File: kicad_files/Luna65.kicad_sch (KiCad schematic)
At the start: 332 parts, among them J1 TYPE-C-31-M12_13, J2 JSTPH, J3 uC Pin Headers, J4 nRF51 Pin Headers, J5 Pin Headers, Q1 DTC123JKAT146, Q2 AO3401A, SW0 SW_Push, SW1 Esc, SW10 9, SW11 0, SW12 -, SW13 =, SW14 BSP_200, SW15 Del, SW16 Tab_150, SW17 Q, SW18 W, SW19 E, SW2 1, SW20 R, SW21 T, SW22 Y, SW23 U, SW24 I, SW25 O, SW26 P, SW27 [, SW28 ], SW29 \_150, SW3 2, SW30 Home, SW31 Caps_175, SW32 A, SW33 S, SW34 D, SW35 F, SW36 G, SW37 H, SW38 J, SW39 K, SW4 3, SW40 L, SW41 ;, SW42 ', SW43 Ent_225, SW44 PgUp, SW45 LShft_225, SW46 Z, SW47 X, SW48 C, SW49 V, SW5 4, SW50 B, SW51 N, SW52 M, SW53 ,, SW54 ., SW55 /, SW56 RShft_175, SW57 Up, SW58 PgDn, SW59 LCtrl_125, SW6 5, SW60 Win_125, SW61 LAlt_125, SW62 Space_625, SW63 RAlt, SW64 Fn, SW65 RCtrl, SW66 Left, SW67 Down, SW68 Right, SW7 6, SW8 7, SW9 8, U1 ATMEGA32U4, U2 USBLC6-2SC6, U3 MCP73831, U4 AP2112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

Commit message: Rev 6 initial changes
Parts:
- removed C1, C8: 4.7nF, acheron_Components:C_0805_2012Metric, symbol Device:C_Small
- removed C10, C9: 10uF, acheron_Components:C_0805_2012Metric, symbol Device:C_Small
- removed C12: 1uF, acheron_Components:C_0805_2012Metric, symbol Device:C_Small
- removed C2: 0.1uF, acheron_Components:C_0805_2012Metric, symbol Device:C_Small
- removed D10, D11, D12, D13, D14, D15, D69, D9: 1N4148W, acheron_Components:D_SOD-123, symbol Device:D_Small
- removed D100, D101, D102, D103, D104, D105, D106, D107, D108, D109, D110, D111, D112, D113, D114, D115, D116, D117, D118, D119, D120, D121, D122, D123, D124, D125, D126, D127, D128, D129, D130, D131, D132, D133, D134, D135, D136, D137, D138, D71, D72, D73, D74, D75, D76, D77, D78, D79, D80, D81, D82, D83, D84, D85, D86, D87, D88, D89, D90, D91, D92, D93, D94, D95, D96, D97, D98, D99: LED_Small, LED_SMD:LED_1206_3216Metric_Pad1.42x1.75mm_HandSolder, symbol Device:LED_Small
- removed D139: Green, LED_SMD:LED_1206_3216Metric_Pad1.42x1.75mm_HandSolder, symbol Device:LED_Small
- removed D70: MBR120, acheron_Components:D_SOD-123, symbol Device:D_Schottky_Small
- removed H4: MountingHole, MountingHole:MountingHole_2.7mm_M2.5_Pad, symbol Mechanical:MountingHole_Pad
- removed J1: TYPE-C-31-M12_13, acheron_Connectors:TYPE-C-31-M-12, symbol acheronSymbols:TYPE-C-31-M12_13
- removed J2: JSTPH, Adafruit Feather 32u4 Bluefruit LE:JSTPH2, symbol Connector_Generic:Conn_01x02
- removed J5: Pin Headers, Connector_PinHeader_1.27mm:PinHeader_2x01_P1.27mm_Vertical, symbol Connector_Generic:Conn_01x02
- removed Q1: DTC123JKAT146, Package_TO_SOT_SMD:SOT-23, symbol acheronSymbols:DTC123J
- removed Q2: AO3401A, Package_TO_SOT_SMD:SOT-23, symbol Transistor_FET:AO3401A
- removed R1, R2: 5.1k, Resistor_SMD:R_0805_2012Metric_Pad1.20x1.40mm_HandSolder, symbol Device:R_Small
- removed R14: 1K, acheron_Components:R_SMD_1206, symbol Device:R
- removed R15: 100, acheron_Components:R_SMD_1206, symbol Device:R
- removed R3: 1M, Resistor_SMD:R_0805_2012Metric_Pad1.20x1.40mm_HandSolder, symbol Device:R_Small
- removed R4, R5: 22, Resistor_SMD:R_0805_2012Metric_Pad1.20x1.40mm_HandSolder, symbol Device:R_Small
- removed R6: 10K, Resistor_SMD:R_0805_2012Metric_Pad1.20x1.40mm_HandSolder, symbol Device:R_Small
- removed R7: 1K, Resistor_SMD:R_0805_2012Metric_Pad1.20x1.40mm_HandSolder, symbol Device:R_Small
- removed R8: 100K, Resistor_SMD:R_0805_2012Metric_Pad1.20x1.40mm_HandSolder, symbol Device:R_Small
- removed R83: 100, acheron_Components:R_SMD_1206, symbol Device:R_Small
- removed R9: 1M, acheron_Components:R_SMD_1206, symbol Device:R_Small
- removed SW10: 9, acheron_MXH:MX100H, symbol acheronSymbols:MXSwitch
- removed SW11: 0, acheron_MXH:MX100H, symbol acheronSymbols:MXSwitch
- removed SW12: -, acheron_MXH:MX100H, symbol acheronSymbols:MXSwitch
- removed SW13: =, acheron_MXH:MX100H, symbol acheronSymbols:MXSwitch
- removed SW14: BSP_200, acheron_MXH:MX200HR, symbol acheronSymbols:MXSwitch
- removed SW15: Del, acheron_MXH:MX100H, symbol acheronSymbols:MXSwitch
- removed SW24: I, acheron_MXH:MX100H, symbol acheronSymbols:MXSwitch
- removed SW25: O, acheron_MXH:MX100H, symbol acheronSymbols:MXSwitch
- removed SW26: P, acheron_MXH:MX100H, symbol acheronSymbols:MXSwitch
- removed SW27: [, acheron_MXH:MX100H, symbol acheronSymbols:MXSwitch
- removed SW28: ], acheron_MXH:MX100H, symbol acheronSymbols:MXSwitch
- removed SW29: \_150, acheron_MXH:MX150H, symbol acheronSymbols:MXSwitch
- removed SW30: Home, acheron_MXH:MX100H, symbol acheronSymbols:MXSwitch
- removed SW39: K, acheron_MXH:MX100H, symbol acheronSymbols:MXSwitch
- removed SW40: L, acheron_MXH:MX100H, symbol acheronSymbols:MXSwitch
- removed SW41: ;, acheron_MXH:MX100H, symbol acheronSymbols:MXSwitch
- removed SW42: ', acheron_MXH:MX100H, symbol acheronSymbols:MXSwitch
- removed SW43: Ent_225, acheron_MXH:MX225HR, symbol acheronSymbols:MXSwitch
- removed SW44: PgUp, acheron_MXH:MX100H, symbol acheronSymbols:MXSwitch
- removed SW52: M, acheron_MXH:MX100H, symbol acheronSymbols:MXSwitch
- removed SW53: ,, acheron_MXH:MX100H, symbol acheronSymbols:MXSwitch
- removed SW54: ., acheron_MXH:MX100H, symbol acheronSymbols:MXSwitch
- removed SW55: /, acheron_MXH:MX100H, symbol acheronSymbols:MXSwitch
- removed SW56: RShft_175, acheron_MXH:MX175H, symbol acheronSymbols:MXSwitch
- removed SW57: Up, acheron_MXH:MX100H, symbol acheronSymbols:MXSwitch
- removed SW58: PgDn, acheron_MXH:MX100H, symbol acheronSymbols:MXSwitch
- removed SW59: LCtrl_125, acheron_MXH:MX125H, symbol acheronSymbols:MXSwitch
- removed SW60: Win_125, acheron_MXH:MX125H, symbol acheronSymbols:MXSwitch
- removed SW61: LAlt_125, acheron_MXH:MX125H, symbol acheronSymbols:MXSwitch
- removed SW62: Space_625, acheron_MXH:MX625H, symbol acheronSymbols:MXSwitch
- removed SW63: RAlt, acheron_MXH:MX100H, symbol acheronSymbols:MXSwitch
- removed SW64: Fn, acheron_MXH:MX100H, symbol acheronSymbols:MXSwitch
- removed SW65: RCtrl, acheron_MXH:MX100H, symbol acheronSymbols:MXSwitch
- removed SW66: Left, acheron_MXH:MX100H, symbol acheronSymbols:MXSwitch
- removed SW67: Down, acheron_MXH:MX100H, symbol acheronSymbols:MXSwitch
- removed SW68: Right, acheron_MXH:MX100H, symbol acheronSymbols:MXSwitch
- removed SW9: 8, acheron_MXH:MX100H, symbol acheronSymbols:MXSwitch
- removed U2: USBLC6-2SC6, Package_TO_SOT_SMD:SOT-23-6, symbol Power_Protection:USBLC6-2SC6
- removed U3: MCP73831, Package_TO_SOT_SMD:SOT-23-5, symbol Battery_Management:MCP73831-2-OT
- removed U4: AP2112, Package_TO_SOT_SMD:SOT-23-5, symbol Regulator_Linear:SPX3819M5-L-3-3
- added C13, C14, C15, C16, C17, C18, C19, C20, C21, C22, C23, C24, C25, C26, C27, C28, C29, C30, C31, C32, C33, C34, C35, C36, C37, C38, C39, C40, C41, C42, C43, C44, C45, C46, C47, C48, C49, C50, C51, C52, C53, C54, C55, C56, C57, C58, C59, C60, C61, C62, C63, C64, C65, C66, C67, C68, C69, C70, C71, C72, C73, C74, C75, C76, C77, C78, C79, C80: 100n, acheron_Components:C_0805_2012Metric, symbol Device:C_Small
- added C81, C82: 100n, acheron_Components:C_0805_2012Metric, symbol Device:C
- added D100, D101, D102, D103, D104, D105, D106, D107, D108, D109, D110, D111, D112, D113, D114, D115, D116, D117, D118, D119, D120, D121, D122, D123, D124, D125, D126, D127, D128, D129, D130, D131, D132, D133, D134, D135, D136, D69, D70, D71, D72, D73, D74, D75, D76, D77, D78, D79, D80, D81, D82, D83, D84, D85, D86, D87, D88, D89, D90, D91, D92, D93, D94, D95, D96, D97, D98, D99: SK6812MINI-E, acheron_Components:SK6812MINI_3535_6028_3.2x2.8mm_Round, symbol acheron_Symbols:SK6812MINI-E
- added D59, D60, D61, D62, D63, D64, D65: 1N4148W, acheron_Components:D_SOD-123, symbol Device:D_Small
- added H4: MountingHole, MountingHole:MountingHole_2.7mm_M2.5_Pad, symbol Mechanical:MountingHole
- added J1: Molex Power, Luna65:MOLEX_78171-0005, symbol Connector_Generic:Conn_01x05
- added R14, R15: 5.1R, acheron_Components:C_0805_2012Metric, symbol Device:R_Small
- added SW24, SW25, SW26, SW27, SW28, SW30, SW32, SW33, SW34, SW35, SW36, SW37, SW38, SW39, SW40, SW41, SW42, SW44, SW53, SW54, SW55, SW57, SW58, SW63, SW64, SW65, SW66, SW67, SW68: Mechanical_Switch, acheron_MXH_metalrings:MX100H, symbol acheron_Symbols:Mechanical_Switch
- added SW29: Mechanical_Switch, acheron_MXH_metalrings:MX150H, symbol acheron_Symbols:Mechanical_Switch
- added SW31, SW56: Mechanical_Switch, acheron_MXH_metalrings:MX175H, symbol acheron_Symbols:Mechanical_Switch
- added SW43: Mechanical_Switch, acheron_MXH_metalrings:MX225H, symbol acheron_Symbols:Mechanical_Switch
- added SW59, SW60, SW61: Mechanical_Switch, acheron_MXH_metalrings:MX125H, symbol acheron_Symbols:Mechanical_Switch
- added SW62: Mechanical_Switch, acheron_MXH_metalrings:MX625HR, symbol acheron_Symbols:Mechanical_Switch
- added U3: TXS0101DBVR, acheron_Components:SOT-23-6, symbol acheronSymbols:TXS0101
- J2: renamed from J3; footprint Connector_PinHeader_1.27mm:PinHeader_2x03_P1.27mm_Vertical -> Connector_PinHeader_2.54mm:PinHeader_2x03_P2.54mm_Vertical
- J3: renamed from J4; footprint Connector_PinHeader_1.27mm:PinHeader_2x03_P1.27mm_Vertical -> Connector_PinHeader_2.54mm:PinHeader_2x03_P2.54mm_Vertical
- R16, R17, R18, R19, R20, R21, R22, R23, R24, R25, R26, R27, R28, R29, R30, R31, R32, R33, R34, R35, R36, R37, R38, R39, R40, R41, R42, R43, R44, R45, R46, R47, R48, R49, R50, R51, R52, R53, R54, R55, R56, R57, R58, R59, R60, R61, R62, R63, R64, R65, R66, R67, R68, R69, R70, R71, R72, R73, R74, R75, R76, R77, R78, R79, R80, R81: value 100 -> 5.1R; footprint acheron_Components:R_SMD_1206 -> acheron_Components:C_0805_2012Metric; Package (none) -> R0402
- R82: value 100 -> 10k; footprint acheron_Components:R_SMD_1206 -> Resistor_SMD:R_0805_2012Metric_Pad1.20x1.40mm_HandSolder; Package (none) -> R0805
- SW1: value Esc -> Mechanical_Switch; footprint acheron_MXH:MX100H -> acheron_MXH_metalrings:MX100H; symbol acheronSymbols:MXSwitch -> acheron_Symbols:Mechanical_Switch; Keycode (none) -> ESC
- SW10: renamed from SW46; value Z -> Mechanical_Switch; footprint acheron_MXH:MX100H -> acheron_MXH_metalrings:MX100H; symbol acheronSymbols:MXSwitch -> acheron_Symbols:Mechanical_Switch; Keycode (none) -> 9
- SW11: renamed from SW47; value X -> Mechanical_Switch; footprint acheron_MXH:MX100H -> acheron_MXH_metalrings:MX100H; symbol acheronSymbols:MXSwitch -> acheron_Symbols:Mechanical_Switch; Keycode (none) -> 0
- SW12: renamed from SW48; value C -> Mechanical_Switch; footprint acheron_MXH:MX100H -> acheron_MXH_metalrings:MX100H; symbol acheronSymbols:MXSwitch -> acheron_Symbols:Mechanical_Switch; Keycode (none) -> -
- SW13: renamed from SW49; value V -> Mechanical_Switch; footprint acheron_MXH:MX100H -> acheron_MXH_metalrings:MX100H; symbol acheronSymbols:MXSwitch -> acheron_Symbols:Mechanical_Switch; Keycode (none) -> =
- SW14: renamed from SW50; value B -> Mechanical_Switch; footprint acheron_MXH:MX100H -> acheron_MXH_metalrings:MX200H; symbol acheronSymbols:MXSwitch -> acheron_Symbols:Mechanical_Switch; Keycode (none) -> BSPC
- SW15: renamed from SW51; value N -> Mechanical_Switch; footprint acheron_MXH:MX100H -> acheron_MXH_metalrings:MX100H; symbol acheronSymbols:MXSwitch -> acheron_Symbols:Mechanical_Switch; Keycode (none) -> HOME
- SW16: value Tab_150 -> Mechanical_Switch; footprint acheron_MXH:MX150H -> acheron_MXH_metalrings:MX150H; symbol acheronSymbols:MXSwitch -> acheron_Symbols:Mechanical_Switch; Keycode (none) -> TAB
- SW17: value Q -> Mechanical_Switch; footprint acheron_MXH:MX100H -> acheron_MXH_metalrings:MX100H; symbol acheronSymbols:MXSwitch -> acheron_Symbols:Mechanical_Switch; Keycode (none) -> Q
- SW18: value W -> Mechanical_Switch; footprint acheron_MXH:MX100H -> acheron_MXH_metalrings:MX100H; symbol acheronSymbols:MXSwitch -> acheron_Symbols:Mechanical_Switch; Keycode (none) -> W
- SW19: value E -> Mechanical_Switch; footprint acheron_MXH:MX100H -> acheron_MXH_metalrings:MX100H; symbol acheronSymbols:MXSwitch -> acheron_Symbols:Mechanical_Switch; Keycode (none) -> E
- SW2: value 1 -> Mechanical_Switch; footprint acheron_MXH:MX100H -> acheron_MXH_metalrings:MX100H; symbol acheronSymbols:MXSwitch -> acheron_Symbols:Mechanical_Switch; Keycode (none) -> 1
- SW20: value R -> Mechanical_Switch; footprint acheron_MXH:MX100H -> acheron_MXH_metalrings:MX100H; symbol acheronSymbols:MXSwitch -> acheron_Symbols:Mechanical_Switch; Keycode (none) -> R
- SW21: value T -> Mechanical_Switch; footprint acheron_MXH:MX100H -> acheron_MXH_metalrings:MX100H; symbol acheronSymbols:MXSwitch -> acheron_Symbols:Mechanical_Switch; Keycode (none) -> T
- SW22: value Y -> Mechanical_Switch; footprint acheron_MXH:MX100H -> acheron_MXH_metalrings:MX100H; symbol acheronSymbols:MXSwitch -> acheron_Symbols:Mechanical_Switch; Keycode (none) -> Y
- SW23: value U -> Mechanical_Switch; footprint acheron_MXH:MX100H -> acheron_MXH_metalrings:MX100H; symbol acheronSymbols:MXSwitch -> acheron_Symbols:Mechanical_Switch; Keycode (none) -> U
- SW3: value 2 -> Mechanical_Switch; footprint acheron_MXH:MX100H -> acheron_MXH_metalrings:MX100H; symbol acheronSymbols:MXSwitch -> acheron_Symbols:Mechanical_Switch; Keycode (none) -> 2
- SW4: value 3 -> Mechanical_Switch; footprint acheron_MXH:MX100H -> acheron_MXH_metalrings:MX100H; symbol acheronSymbols:MXSwitch -> acheron_Symbols:Mechanical_Switch; Keycode (none) -> 3
- SW45: renamed from SW31; value Caps_175 -> Mechanical_Switch; footprint acheron_MXH:MX175H -> acheron_MXH_metalrings:MX225H; symbol acheronSymbols:MXSwitch -> acheron_Symbols:Mechanical_Switch; Keycode (none) -> LSHFT
- SW46: renamed from SW32; value A -> Mechanical_Switch; footprint acheron_MXH:MX100H -> acheron_MXH_metalrings:MX100H; symbol acheronSymbols:MXSwitch -> acheron_Symbols:Mechanical_Switch; Keycode (none) -> Z
- SW47: renamed from SW33; value S -> Mechanical_Switch; footprint acheron_MXH:MX100H -> acheron_MXH_metalrings:MX100H; symbol acheronSymbols:MXSwitch -> acheron_Symbols:Mechanical_Switch; Keycode (none) -> X
- SW48: renamed from SW34; value D -> Mechanical_Switch; footprint acheron_MXH:MX100H -> acheron_MXH_metalrings:MX100H; symbol acheronSymbols:MXSwitch -> acheron_Symbols:Mechanical_Switch; Keycode (none) -> C
- SW49: renamed from SW35; value F -> Mechanical_Switch; footprint acheron_MXH:MX100H -> acheron_MXH_metalrings:MX100H; symbol acheronSymbols:MXSwitch -> acheron_Symbols:Mechanical_Switch; Keycode (none) -> V
- SW5: value 4 -> Mechanical_Switch; footprint acheron_MXH:MX100H -> acheron_MXH_metalrings:MX100H; symbol acheronSymbols:MXSwitch -> acheron_Symbols:Mechanical_Switch; Keycode (none) -> 4
- SW50: renamed from SW36; value G -> Mechanical_Switch; footprint acheron_MXH:MX100H -> acheron_MXH_metalrings:MX100H; symbol acheronSymbols:MXSwitch -> acheron_Symbols:Mechanical_Switch; Keycode (none) -> B
- SW51: renamed from SW37; value H -> Mechanical_Switch; footprint acheron_MXH:MX100H -> acheron_MXH_metalrings:MX100H; symbol acheronSymbols:MXSwitch -> acheron_Symbols:Mechanical_Switch; Keycode (none) -> N
- SW52: renamed from SW38; value J -> Mechanical_Switch; footprint acheron_MXH:MX100H -> acheron_MXH_metalrings:MX100H; symbol acheronSymbols:MXSwitch -> acheron_Symbols:Mechanical_Switch; Keycode (none) -> M
- SW6: value 5 -> Mechanical_Switch; footprint acheron_MXH:MX100H -> acheron_MXH_metalrings:MX100H; symbol acheronSymbols:MXSwitch -> acheron_Symbols:Mechanical_Switch; Keycode (none) -> 5
- SW7: value 6 -> Mechanical_Switch; footprint acheron_MXH:MX100H -> acheron_MXH_metalrings:MX100H; symbol acheronSymbols:MXSwitch -> acheron_Symbols:Mechanical_Switch; Keycode (none) -> 6
- SW8: value 7 -> Mechanical_Switch; footprint acheron_MXH:MX100H -> acheron_MXH_metalrings:MX100H; symbol acheronSymbols:MXSwitch -> acheron_Symbols:Mechanical_Switch; Keycode (none) -> 7
- SW9: renamed from SW45; value LShft_225 -> Mechanical_Switch; footprint acheron_MXH:MX225HR -> acheron_MXH_metalrings:MX100H; symbol acheronSymbols:MXSwitch -> acheron_Symbols:Mechanical_Switch; Keycode (none) -> 8
- Y1: value 8MHz -> 16MHz
- renumbered C13 to C11, D60 to D10, D61 to D11, D62 to D12, D63 to D13, D140 to D137, D141 to D138, D64 to D14, D65 to D15, D59 to D9, U5 to U2
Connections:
- net LED_PWM is gone; now on net Row1: U1.18 (PD0/SCL/~{INT0})
- net VBUS is gone; now on net 5V: U1.7 (VBUS)
- net 3.3V: now also J2.5 (Pin_5), R82.1, C81.2, J1.1 (Pin_1), U3.1 (VCCA); no longer J2.2 (Pin_2)
- net Col1: now also U1.26 (ADC9/T1/PD6), SW31.1, SW59.1; no longer SW9.1 (Col), U1.36 (ADC7/PF7)
- net Col10: now also SW10.1, U1.38 (ADC5/PF5), SW25.1, SW40.1, SW54.1, SW58.1, SW64.1; no longer U1.31 (PC6)
- net Col11: now also SW11.1, U1.39 (ADC4/PF4), SW26.1, SW41.1, SW55.1, SW65.1, SW68.1; no longer U1.30 (PCINT6/ADC13/PB6)
- net Col12: now also SW12.1, U1.40 (ADC1/PF1), SW27.1, SW42.1, SW56.1, SW66.1, SW67.1; no longer U1.29 (PCINT4/ADC12/PB5)
- net Col2: now also U1.27 (ADC10/T0/PD7), SW32.1, SW60.1; no longer SW10.1 (Col), U1.19 (PD1/SDA/~{INT1})
- net Col3: now also U1.28 (ADC4/PCINT11/PB4), SW33.1, SW61.1; no longer SW11.1 (Col), U1.20 (PD2/RDX1/~{INT2})
- net Col4: now also U1.29 (PCINT4/ADC12/PB5), SW34.1, SW62.1; no longer SW12.1 (Col), U1.21 (PD3/TXD1/~{INT3})
- net Col5: now also U1.30 (PCINT6/ADC13/PB6), SW35.1, SW43.1, SW44.1; no longer SW13.1 (Col), U1.22 (PD5/~{CTS}/XCK1)
- net Col6: now also SW15.1, U1.31 (PC6), SW30.1, SW36.1; no longer SW14.1 (Col), U1.26 (ADC9/T1/PD6)
- net Col7: now also SW14.1, U1.32 (CLK/PC7), SW29.1, SW37.1; no longer SW15.1 (Col), U1.27 (ADC10/T0/PD7)
- net Col8: now also SW13.1, U1.36 (ADC7/PF7), SW28.1, SW38.1; no longer U1.12 (PB7/RTS)
- net Col9: now also SW9.1, U1.37 (ADC6/PF6), SW24.1, SW39.1, SW53.1, SW57.1, SW63.1; no longer U1.32 (CLK/PC7)
- net D+: now also J1.4 (Pin_4)
- net D-: now also J1.3 (Pin_3)
- net GND: now also C13.2, C14.2, C15.2, C16.2, C17.2, C18.2, C19.2, C20.2, C21.2, C22.2, C23.2, C24.2, C25.2, C26.2, C27.2, C28.2, C29.2, C30.2, C31.2, C32.2, C33.2, C34.2, C35.2, C36.2, C37.2, C38.2, C39.2, C40.2, C41.2, C42.2, C43.2, C44.2, C45.2, C46.2, C47.2, C48.2, C49.2, C50.2, C51.2, C52.2, C53.2, C54.2, C55.2, C56.2, C57.2, C58.2, C59.2, C60.2, C61.2, C62.2, C63.2, C64.2, C65.2, C66.2, C67.2, C68.2, C69.2, C70.2, C71.2, C72.2, C73.2, C74.2, C75.2, C76.2, C77.2, C78.2, C79.2, C80.2, C81.1, C82.2, D100.3 (VSS), D101.3 (VSS), D102.3 (VSS), D103.3 (VSS), D104.3 (VSS), D105.3 (VSS), D106.3 (VSS), D107.3 (VSS), D108.3 (VSS), D109.3 (VSS), D110.3 (VSS), D111.3 (VSS), D112.3 (VSS), D113.3 (VSS), D114.3 (VSS), D115.3 (VSS), D116.3 (VSS), D117.3 (VSS), D118.3 (VSS), D119.3 (VSS), D120.3 (VSS), D121.3 (VSS), D122.3 (VSS), D123.3 (VSS), D124.3 (VSS), D125.3 (VSS), D126.3 (VSS), D127.3 (VSS), D128.3 (VSS), D129.3 (VSS), D130.3 (VSS), D131.3 (VSS), D132.3 (VSS), D133.3 (VSS), D134.3 (VSS), D135.3 (VSS), D136.3 (VSS), D69.3 (VSS), D70.3 (VSS), D71.3 (VSS), D72.3 (VSS), D73.3 (VSS), D74.3 (VSS), D75.3 (VSS), D76.3 (VSS), D77.3 (VSS), D78.3 (VSS), D79.3 (VSS), D80.3 (VSS), D81.3 (VSS), D82.3 (VSS), D83.3 (VSS), D84.3 (VSS), D85.3 (VSS), D86.3 (VSS), D87.3 (VSS), D88.3 (VSS), D89.3 (VSS), D90.3 (VSS), D91.3 (VSS), D92.3 (VSS), D93.3 (VSS), D94.3 (VSS), D95.3 (VSS), D96.3 (VSS), D97.3 (VSS), D98.3 (VSS), D99.3 (VSS), J1.5 (Pin_5), U3.2 (GND)
- net MISO: now also J2.3 (Pin_3); no longer J2.1 (Pin_1)
- net MOSI: now also J2.1 (Pin_1); no longer J2.4 (Pin_4)
- net RESET: now also J2.2 (Pin_2); no longer J2.5 (Pin_5)
- net Row1: now also D10.1 (K), D11.1 (K), D12.1 (K), D9.1 (K); no longer U1.41 (ADC0/PF0)
- net Row2: now also U1.19 (PD1/SDA/~{INT1}); no longer U1.40 (ADC1/PF1)
- net Row3: now also U1.20 (PD2/RDX1/~{INT2}); no longer U1.39 (ADC4/PF4)
- net Row4: now also U1.22 (PD5/~{CTS}/XCK1); no longer U1.38 (ADC5/PF5)
- net Row5: now also D28.1 (K), D29.1 (K), D30.1 (K), D43.1 (K), U1.21 (PD3/TXD1/~{INT3}), D59.1 (K), D60.1 (K), D61.1 (K), D62.1 (K), D63.1 (K), D64.1 (K), D65.1 (K); no longer D10.1 (K), D11.1 (K), D12.1 (K), D13.1 (K), D14.1 (K), D15.1 (K), D44.1 (K), D58.1 (K), D67.1 (K), D68.1 (K), D9.1 (K), U1.37 (ADC6/PF6)
- net Row6: now also D13.1 (K), D14.1 (K), D15.1 (K), D44.1 (K), D58.1 (K), D67.1 (K), D68.1 (K), U1.41 (ADC0/PF0); no longer D28.1 (K), D29.1 (K), D30.1 (K), D43.1 (K), U1.28 (ADC4/PCINT11/PB4)
- net SCK: now also J2.4 (Pin_4); no longer J2.3 (Pin_3)
- net at SW14.2: now also D14.2 (A); no longer D50.2 (A)
- net 5V: now reaches R73.2
- net 5V: now also R16.2, R17.2, R18.2, R19.2, R20.2, R21.2, R22.2, R23.2, R24.2, R25.2, R26.2, R27.2, R28.2, R29.2, R30.2, R31.2, R32.2, R33.2, R34.2, R35.2, R36.2, R37.2, R38.2, R39.2, R40.2, R41.2, R42.2, R43.2, R44.2, R45.2, R46.2, R47.2, R48.2, R49.2, R50.2, R51.2, R52.2, R53.2, R54.2, R55.2, R56.2, R57.2, R58.2, R59.2, R60.2, R61.2, R62.2, R63.2, R64.2, R65.2, R66.2, R67.2, R68.2, R69.2, R70.2, R71.2, R72.2, R74.2, R75.2, R76.2, R77.2, R78.2, R79.2, R80.2, R81.2, C82.1, J1.2 (Pin_2), R14.2, R15.2, U3.6 (VCCB)
- net at SW52.2: now also D52.2 (A); no longer D38.2 (A)
- net at D42.2 (A): now also SW42.2
- net at D58.2 (A): now also SW58.2
- net at SW50.2: now also D50.2 (A); no longer D36.2 (A)
- net at SW10.2: now also D10.2 (A); no longer D46.2 (A)
- net at R82.2: now also U3.5 (OE)
- net at D15.2 (A): now also SW15.2
- net at D12.2 (A): now also SW12.2
- net at D31.2 (A): now also SW31.2; no longer SW45.2 (Row)
- net at D66.2 (A): now also SW66.2
- net at D26.2 (A): now also SW26.2
- net at SW48.2: now also D48.2 (A); no longer D34.2 (A)
- net at D43.2 (A): now also SW43.2
- net at SW51.2: now also D51.2 (A); no longer D37.2 (A)
- net at D55.2 (A): now also SW55.2
- net at D40.2 (A): now also SW40.2
- net at D25.2 (A): now also SW25.2
- net at D67.2 (A): now also SW67.2
- net at D30.2 (A): now also SW30.2
- net at SW46.2: now also D46.2 (A); no longer D32.2 (A)
- net at D11.2 (A): now also SW11.2
- net at D29.2 (A): now also SW29.2
- net at D49.2 (A): now also SW49.2; no longer SW13.2 (Row)
- net at D54.2 (A): now also SW54.2
- net at D47.2 (A): now also SW47.2; no longer SW11.2 (Row)
- net at D9.2 (A): now also SW9.2
- net at D13.2 (A): now also SW13.2
- net at D28.2 (A): now also SW28.2
- net at D35.2 (A): now also SW35.2; no longer SW49.2 (Row)
- net at D53.2 (A): now also SW53.2
- net at D68.2 (A): now also SW68.2
- net at D45.2 (A): now also SW45.2; no longer SW9.2 (Row)
- net at D24.2 (A): now also SW24.2
- net at D39.2 (A): now also SW39.2
- net at D44.2 (A): now also SW44.2
- net at D27.2 (A): now also SW27.2
- net at D57.2 (A): now also SW57.2
- net at D56.2 (A): now also SW56.2
- net at D41.2 (A): now also SW41.2
- net at D33.2 (A): now also SW33.2; no longer SW47.2 (Row)
- new net: C21.1, D77.1 (VDD), R22.1
- new net: C13.1, D69.1 (VDD), R14.1
- new net: C41.1, D97.1 (VDD), R42.1
- new net: C52.1, D108.1 (VDD), R53.1
- new net: C33.1, D89.1 (VDD), R34.1
- new net: D60.2 (A), SW60.2
- new net: C67.1, D123.1 (VDD), R68.1
- new net: D119.4 (DIN), D123.2 (DOUT)
- new net: D123.4 (DIN), D127.2 (DOUT)
- new net: C64.1, D120.1 (VDD), R65.1
- new net: C28.1, D84.1 (VDD), R29.1
- new net: C16.1, D72.1 (VDD), R17.1
- new net: C42.1, D98.1 (VDD), R43.1
- new net: C15.1, D129.1 (VDD), R16.1
- new net: D65.2 (A), SW65.2
- new net: C26.1, D82.1 (VDD), R27.1
- new net: D82.2 (DOUT), D87.4 (DIN)
- new net: D77.2 (DOUT), D82.4 (DIN)
- new net: C74.1, D130.1 (VDD), R75.1
- new net: C69.1, D116.1 (VDD), R70.1
- new net: D111.4 (DIN), D116.2 (DOUT)
- new net: D116.4 (DIN), D121.2 (DOUT)
- new net: D84.4 (DIN), D89.2 (DOUT)
- new net: D89.4 (DIN), D94.2 (DOUT)
- new net: C37.1, D93.1 (VDD), R38.1
- new net: C32.1, D88.1 (VDD), R33.1
- new net: D83.4 (DIN), D88.2 (DOUT)
- new net: D88.4 (DIN), D93.2 (DOUT)
- new net: C55.1, D101.1 (VDD), R56.1
- new net: D101.2 (DOUT), D96.4 (DIN)
- new net: D101.4 (DIN), D106.2 (DOUT)
- new net: D62.2 (A), SW62.2
- new net: C36.1, D92.1 (VDD), R37.1
- new net: D63.2 (A), SW63.2
- new net: C73.1, D121.1 (VDD), R74.1
- new net: C35.1, D81.1 (VDD), R36.1
- new net: C66.1, D122.1 (VDD), R67.1
- new net: C54.1, D110.1 (VDD), R55.1
- new net: C57.1, D113.1 (VDD), R58.1
- new net: C40.1, D86.1 (VDD), R41.1
- new net: D81.4 (DIN), D86.2 (DOUT)
- new net: D86.4 (DIN), D91.2 (DOUT)
- new net: D92.2 (DOUT), D97.4 (DIN)
- new net: D87.2 (DOUT), D92.4 (DIN)
- new net: D64.2 (A), SW64.2
- new net: D59.2 (A), SW59.2
- new net: C75.1, D131.1 (VDD), R76.1
- new net: D127.4 (DIN), D131.2 (DOUT)
- new net: D131.4 (DIN), D135.2 (DOUT)
- new net: C18.1, D74.1 (VDD), R19.1
- new net: C61.1, D117.1 (VDD), R62.1
- new net: C49.1, D105.1 (VDD), R50.1
- new net: D105.2 (DOUT), D110.4 (DIN)
- new net: D100.2 (DOUT), D105.4 (DIN)
- new net: C76.1, D132.1 (VDD), R77.1
- new net: C65.1, D111.1 (VDD), R66.1
- new net: D106.4 (DIN), D111.2 (DOUT)
- new net: C70.1, D126.1 (VDD), R71.1
- new net: C38.1, D94.1 (VDD), R39.1
- new net: C51.1, D107.1 (VDD), R52.1
- new net: D107.2 (DOUT), D112.4 (DIN)
- new net: D102.2 (DOUT), D107.4 (DIN)
- new net: C22.1, D78.1 (VDD), R23.1
- new net: C59.1, D115.1 (VDD), R60.1
- new net: D69.4 (DIN), D74.2 (DOUT)
- new net: D74.4 (DIN), D79.2 (DOUT)
- new net: C45.1, D91.1 (VDD), R46.1
- new net: D110.2 (DOUT), D115.4 (DIN)
- new net: D61.2 (A), SW61.2
- new net: D120.2 (DOUT), D124.4 (DIN)
- new net: D115.2 (DOUT), D120.4 (DIN)
- new net: D129.2 (DOUT), D70.4 (DIN)
- new net: D129.4 (DIN), D133.2 (DOUT)
- new net: C58.1, D114.1 (VDD), R59.1
- new net: D94.4 (DIN), D99.2 (DOUT)
- new net: C27.1, D83.1 (VDD), R28.1
- new net: C60.1, D106.1 (VDD), R61.1
- new net: D122.2 (DOUT), D126.4 (DIN)
- new net: D117.2 (DOUT), D122.4 (DIN)
- new net: C47.1, D103.1 (VDD), R48.1
- new net: C56.1, D112.1 (VDD), R57.1
- new net: C17.1, D73.1 (VDD), R18.1
- new net: C79.1, D135.1 (VDD), R80.1
- new net: C25.1, D71.1 (VDD), R26.1
- new net: C78.1, D134.1 (VDD), R79.1
- new net: C23.1, D79.1 (VDD), R24.1
- new net: D79.4 (DIN), D84.2 (DOUT)
- new net: C44.1, D100.1 (VDD), R45.1
- new net: D100.4 (DIN), D95.2 (DOUT)
- new net: D135.4 (DIN), D136.2 (DOUT)
- new net: D72.2 (DOUT), D77.4 (DIN)
- new net: D72.4 (DIN), D73.2 (DOUT)
- new net: C63.1, D119.1 (VDD), R64.1
- new net: C48.1, D104.1 (VDD), R49.1
- new net: C77.1, D125.1 (VDD), R78.1
- new net: D121.4 (DIN), D125.2 (DOUT)
- new net: D125.4 (DIN), D134.2 (DOUT)
- new net: C39.1, D95.1 (VDD), R40.1
- new net: C20.1, D133.1 (VDD), R21.1
- new net: D133.4 (DIN), D71.2 (DOUT)
- new net: D36.2 (A), SW36.2
- new net: D112.2 (DOUT), D117.4 (DIN)
- new net: D93.4 (DIN), D98.2 (DOUT)
- new net: D103.2 (DOUT), D98.4 (DIN)
- new net: D37.2 (A), SW37.2
- new net: D102.4 (DIN), D97.2 (DOUT)
- new net: D132.2 (DOUT), D136.4 (DIN)
- new net: D128.2 (DOUT), D132.4 (DIN)
- new net: D109.4 (DIN), D114.2 (DOUT)
- new net: D114.4 (DIN), D119.2 (DOUT)
- new net: D73.4 (DIN), D78.2 (DOUT)
- new net: D38.2 (A), SW38.2
- new net: D130.2 (DOUT), D134.4 (DIN)
- new net: D126.2 (DOUT), D130.4 (DIN)
- new net: C46.1, D102.1 (VDD), R47.1
- new net: C71.1, D127.1 (VDD), R72.1
- new net: C50.1, D96.1 (VDD), R51.1
- new net: C62.1, D118.1 (VDD), R63.1
- new net: D103.4 (DIN), D108.2 (DOUT)
- new net: D78.4 (DIN), D83.2 (DOUT)
- new net: C53.1, D109.1 (VDD), R54.1
- new net: D108.4 (DIN), D113.2 (DOUT)
- new net: D34.2 (A), SW34.2
- new net: C72.1, D128.1 (VDD), R73.1
- new net: C24.1, D80.1 (VDD), R25.1
- new net: D104.2 (DOUT), D99.4 (DIN)
- new net: D104.4 (DIN), D109.2 (DOUT)
- new net: C80.1, D136.1 (VDD), R81.1
- new net: C14.1, D70.1 (VDD), R15.1
- new net: D90.2 (DOUT), D95.4 (DIN)
- new net: C68.1, D124.1 (VDD), R69.1
- new net: C43.1, D99.1 (VDD), R44.1
- new net: C31.1, D87.1 (VDD), R32.1
- new net: D113.4 (DIN), D118.2 (DOUT)
- new net: D76.4 (DIN), D81.2 (DOUT)
- new net: D91.4 (DIN), D96.2 (DOUT)
- new net: C29.1, D85.1 (VDD), R30.1
- new net: D85.2 (DOUT), D90.4 (DIN)
- new net: D80.2 (DOUT), D85.4 (DIN)
- new net: D70.2 (DOUT), D75.4 (DIN)
- new net: C30.1, D76.1 (VDD), R31.1
- new net: D71.4 (DIN), D76.2 (DOUT)
- new net: C19.1, D75.1 (VDD), R20.1
- new net: D124.2 (DOUT), D128.4 (DIN)
- new net: D75.2 (DOUT), D80.4 (DIN)
- new net: C34.1, D90.1 (VDD), R35.1
- new net: D32.2 (A), SW32.2
- new net RGB_3V3: U1.12 (PB7/RTS), U3.3 (A)
- new net RGB_5V: D118.4 (DIN), U3.4 (B)
- no-connect marks 4 -> 2
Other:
- note added: "'"
- note added: ","
- note added: "-"
- note added: "."
- note added: "/"
- note added: "0"
- note added: "16 February 2022"
- note added: "2"
- note added: "3"
- note added: "4"
- note added: "6"
- note added: "7"
- note added: "8"
- note added: "9"
- note added: ":"
- note added: "="
- note added: "A"
- note added: "B"
- note added: "BKSP"
- note added: "C"
- note added: "CAPS"
- note added: "D"
- note added: "DOWN"
- note added: "Daughter-board connector"
- note added: "E"
- note added: "END"
- note added: "ENT"
- note added: "ESC"
- note added: "F"
- note added: "FN"
- note added: "G"
- note added: "H"
- note added: "HOME"
- note added: "I"
- note added: "J"
- note added: "K"
- note added: "L"
- note added: "LALT"
- note added: "LCTRL"
- note added: "LEFT"
- note added: "LSHFT"
- note added: "M"
- note added: "N"
- note added: "O"
- note added: "P"
- note added: "PGDN"
- note added: "PGUP"
- note added: "Pin Headers"
- note added: "Q"
- note added: "R"
- note added: "RALT"
- note added: "RCTRL"
- note added: "RGB Level Shifter"
- note added: "RGB Matrix"
- note added: "RIGHT"
- note added: "RSHFT"
- note added: "S"
- note added: "SPACE"
- note added: "T"
- note added: "TAB"
- note added: "U"
- note added: "UP"
- note added: "V"
- note added: "W"
- note added: "WIN"
- note added: "X"
- note added: "Y"
- note added: "Z"
- note added: "["
- note added: "\"
- note added: "]"
- note removed: "3.3V LDO Regulator"
- note removed: "7 December 2021"
- note removed: "CASE to GND"
- note removed: "LED Matrix"
- note removed: "LiPo Charge Controller"
- note removed: "Shield"
- note removed: "USB ESD Protection"
- note removed: "USB-C Receptacle"
- moved on the sheet: C11, C3, C4, C5, C6, C7, D1, D10, D11, D12, D13, D137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

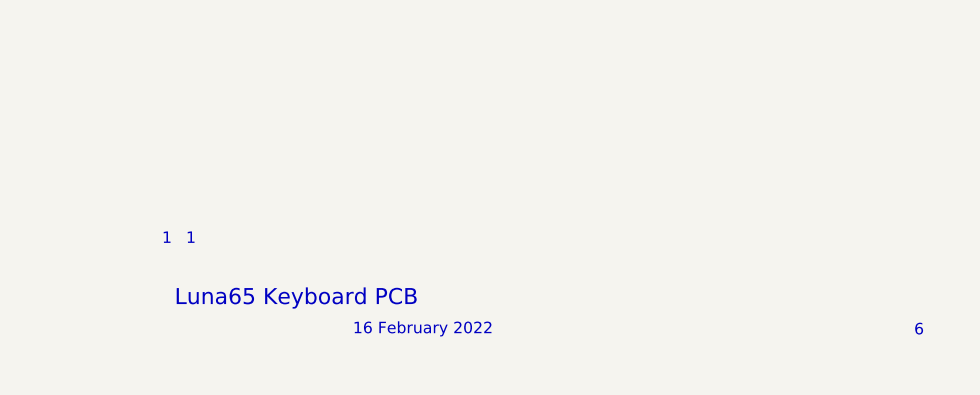
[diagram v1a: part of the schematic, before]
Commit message: DB Rev C
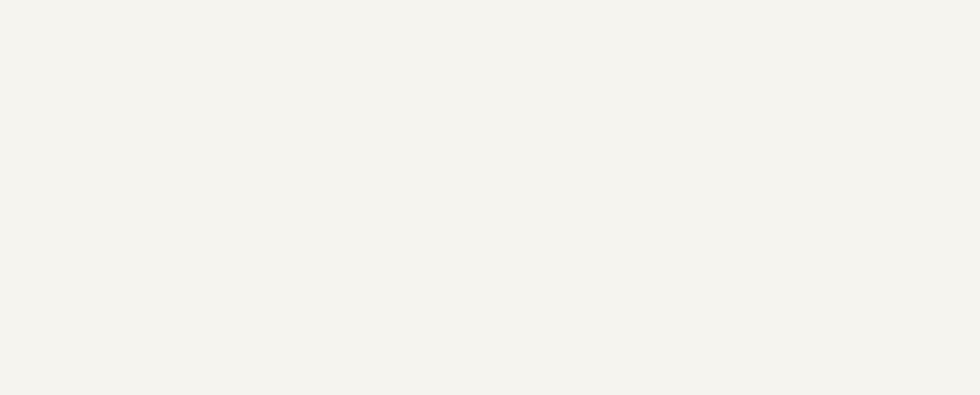
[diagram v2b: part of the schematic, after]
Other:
- note removed: "16 February 2022"
- note removed: "Luna65 Keyboard PCB"
- company: (none) -> Neil Khera
- title: (none) -> Luna65 Keyboard PCB
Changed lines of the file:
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@@
 (kicad_sch (version 20211123) (generator eeschema)
   (paper "User" 799.998 264.998)
+  (title_block
+    (title "Luna65 Keyboard PCB")
+    (date "2022-03-04")
+    (rev "6")
+    (company "Neil Khera")
+  )
   (junction (at 181.356 76.581) (diameter 0) (color 0 0 0 0)
   )
@@
     (effects (font (size 1.27 1.27)) (justify left bottom))
   )
-  (text "6" (at 771.525 249.428 0)
-    (effects (font (size 1.27 1.27)) (justify left bottom))
-  )
   (text "R" (at 533.4 90.551 0)
     (effects (font (size 1.27 1.27)) (justify left bottom))
@@
     (effects (font (size 1.27 1.27)) (justify left bottom))
   )
-  (text "16 February 2022" (at 709.168 249.301 0)
-    (effects (font (size 1.27 1.27)) (justify left bottom))
-  )
   (text "I" (at 625.729 90.551 0)
     (effects (font (size 1.27 1.27)) (justify left bottom))
@@
     (effects (font (size 1.27 1.27)) (justify left bottom))
   )
-  (text "1" (at 687.959 239.268 0)
-    (effects (font (size 1.27 1.27)) (justify left bottom))
-  )
   (text "LSHFT" (at 440.69 179.451 0)
     (effects (font (size 1.27 1.27)) (justify left bottom))
@@
     (effects (font (size 1.27 1.27)) (justify left bottom))
   )
-  (text "1" (at 690.626 239.268 0)
-    (effects (font (size 1.27 1.27)) (justify left bottom))
-  )
-  (text "Luna65 Keyboard PCB\n" (at 689.356 246.126 0)
-    (effects (font (size 1.778 1.778)) (justify left bottom))
-  )
   (text "RGB Matrix" (at 412.75 17.653 0)
